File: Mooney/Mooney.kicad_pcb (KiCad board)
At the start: 2 copper layers, 80.4 x 30.3 mm, 1 part

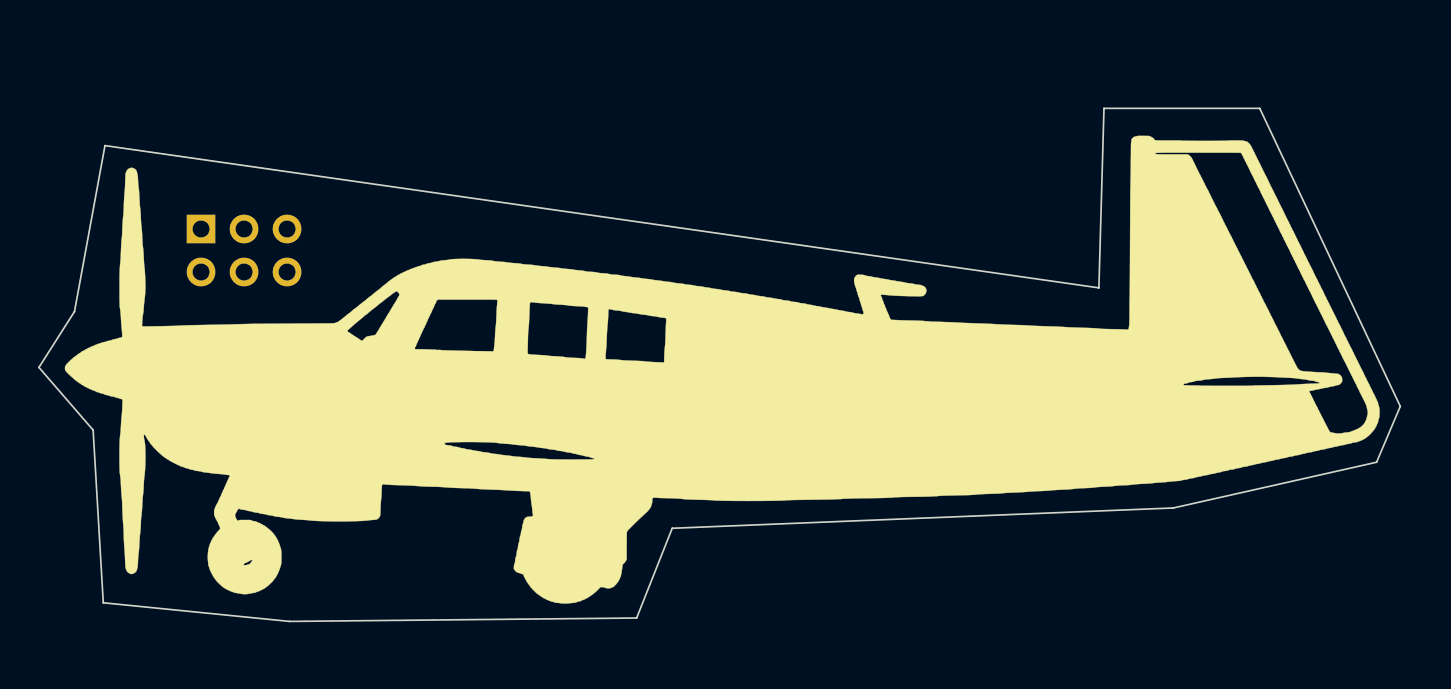
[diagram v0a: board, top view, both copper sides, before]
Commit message: updates to Mooney SAO
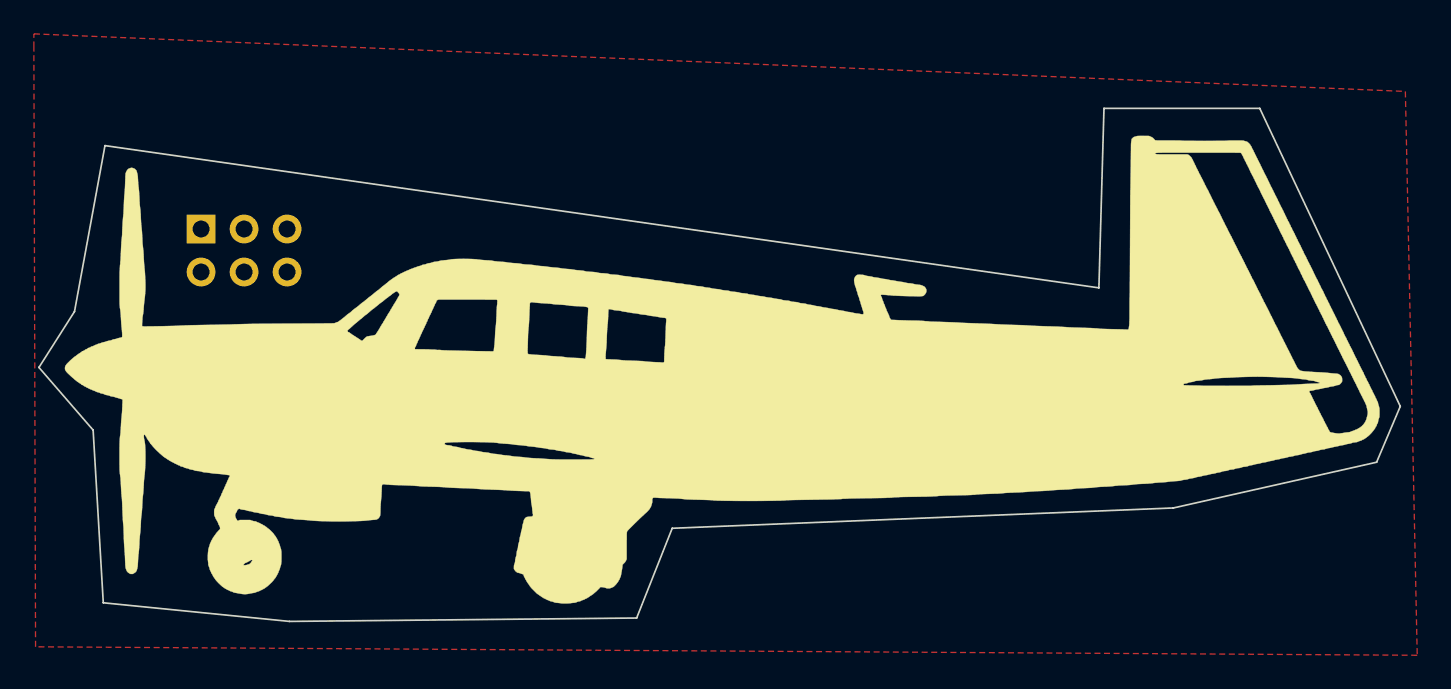
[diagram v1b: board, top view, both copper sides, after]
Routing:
- added copper zone on F.Cu, net (none)
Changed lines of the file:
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@@
-(kicad_pcb (version 20220427) (generator pcbnew)
+(kicad_pcb (version 20220621) (generator pcbnew)
   (general
     (thickness 1.6)
@@
       (usegerberextensions true)
       (usegerberattributes true)
-      (usegerberadvancedattributes true)
+      (usegerberadvancedattributes false)
       (creategerberjobfile false)
       (dashed_line_dash_ratio 12.000000)
@@
     (effects (font (size 1 1) (thickness 0.15)) (justify mirror))
   )
+  (zone (net 0) (net_name "") (layer "F.Cu") (hatch edge 0.508)
+    (connect_pads (clearance 0.508))
+    (min_thickness 0.254) (filled_areas_thickness no)
+    (fill yes (thermal_gap 0.508) (thermal_bridge_width 0.508) (island_removal_mode 2) (island_area_min 10))
+    (polygon
+      (pts
+        (xy 140.1 28.9)
+        (xy 140.8 62.2)
+        (xy 59.2 61.7)
+        (xy 59.1 26.3)
+        (xy 59.1 25.5)
+      )
+    )
+  )
   (group "" (id e30d0bd9-d605-4366-b852-d1e45c1d6a97)
